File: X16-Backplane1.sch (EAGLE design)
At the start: 29 parts, among them J1 CONN_PXC-8-RA-1778683, J12 282837-3, J13 282837-3, J2 CONN_ET60S-D04-3-08-D04-X-R1-S, J3 HTST-110-04-L-D-RA, J4 CLT-110-01-F-D, U2 TRANS_ULN2003AD

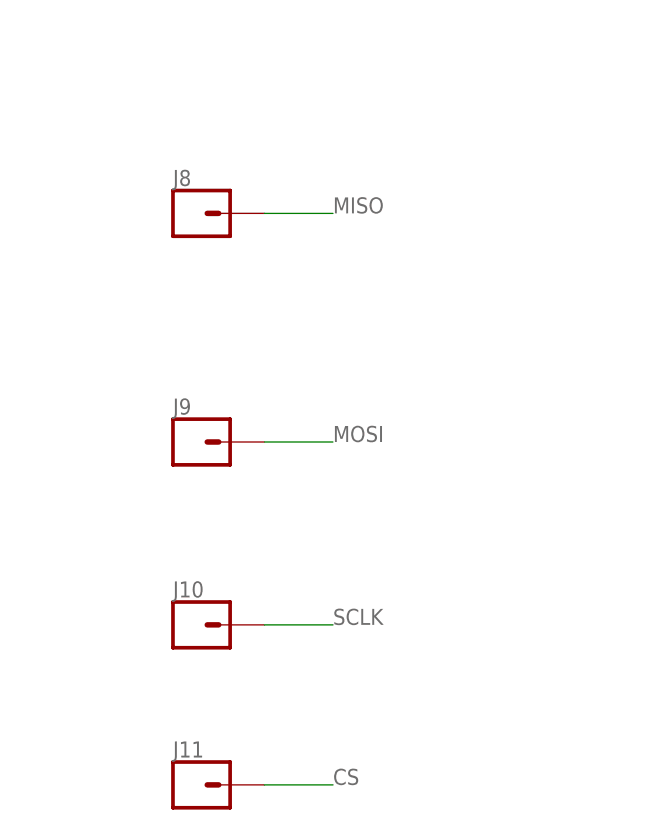
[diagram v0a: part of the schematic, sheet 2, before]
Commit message: Minh Update 3
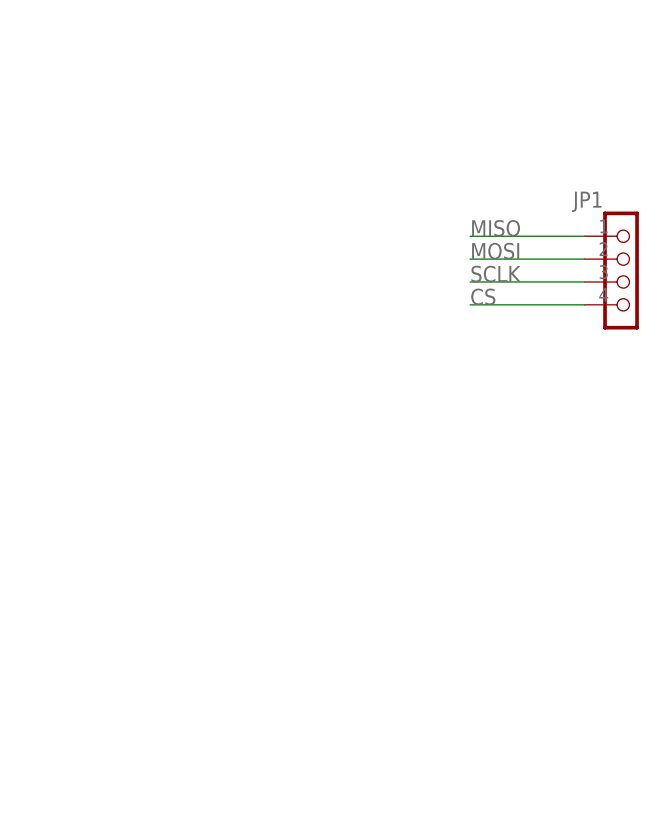
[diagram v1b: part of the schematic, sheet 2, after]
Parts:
- removed J10, J11, J8, J9: (no value), SparkFun-Connectors:CONN_01
- added JP1: (no value), X16-ExtraComponents:TEST_PIN-1X4
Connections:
- net CS: now also JP1.4; no longer J11.1
- net MISO: now also JP1.1; no longer J8.1
- net MOSI: now also JP1.2; no longer J9.1
- net SCLK: now also JP1.3; no longer J10.1
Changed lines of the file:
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@@
 <part name="J3" library="X16_Backplane" deviceset="HTST-110-04-L-D-RA" device=""/>
 <part name="J4" library="X16_Backplane" deviceset="CLT-110-01-F-D" device=""/>
-<part name="J8" library="SparkFun-Connectors" library_urn="urn:adsk.eagle:library:513" deviceset="CONN_01" device="" package3d_urn="urn:adsk.eagle:package:38028/2"/>
-<part name="J9" library="SparkFun-Connectors" library_urn="urn:adsk.eagle:library:513" deviceset="CONN_01" device="" package3d_urn="urn:adsk.eagle:package:38028/2"/>
-<part name="J10" library="SparkFun-Connectors" library_urn="urn:adsk.eagle:library:513" deviceset="CONN_01" device="" package3d_urn="urn:adsk.eagle:package:38028/2"/>
-<part name="J11" library="SparkFun-Connectors" library_urn="urn:adsk.eagle:library:513" deviceset="CONN_01" device="" package3d_urn="urn:adsk.eagle:package:38028/2"/>
 <part name="J12" library="X16_Backplane" deviceset="282837-3" device=""/>
 <part name="J13" library="X16_Backplane" deviceset="282837-3" device=""/>
@@
 <part name="H3" library="X16-ExtraComponents" deviceset="6-32-HOLE" device=""/>
 <part name="H4" library="X16-ExtraComponents" deviceset="6-32-HOLE" device=""/>
+<part name="JP1" library="X16-ExtraComponents" deviceset="TEST_PIN-1X4" device="" package3d_urn="urn:adsk.eagle:package:22407/2"/>
 </parts>
 <sheets>
@@
 <attribute name="C3" x="106.68" y="119.38" size="1.778" layer="96"/>
 </instance>
-<instance part="J8" gate="J1" x="304.8" y="129.54" smashed="yes">
-<attribute name="VALUE" x="302.26" y="124.714" size="1.778" layer="96" font="vector"/>
-<attribute name="NAME" x="302.26" y="132.588" size="1.778" layer="95" font="vector"/>
-</instance>
-<instance part="J9" gate="J1" x="304.8" y="104.14" smashed="yes">
-<attribute name="VALUE" x="302.26" y="99.314" size="1.778" layer="96" font="vector"/>
-<attribute name="NAME" x="302.26" y="107.188" size="1.778" layer="95" font="vector"/>
-</instance>
-<instance part="J10" gate="J1" x="304.8" y="83.82" smashed="yes">
-<attribute name="VALUE" x="302.26" y="78.994" size="1.778" layer="96" font="vector"/>
-<attribute name="NAME" x="302.26" y="86.868" size="1.778" layer="95" font="vector"/>
-</instance>
-<instance part="J11" gate="J1" x="304.8" y="66.04" smashed="yes">
-<attribute name="VALUE" x="302.26" y="61.214" size="1.778" layer="96" font="vector"/>
-<attribute name="NAME" x="302.26" y="69.088" size="1.778" layer="95" font="vector"/>
-</instance>
 <instance part="J12" gate="G$1" x="210.82" y="215.9" smashed="yes">
 <attribute name="NAME" x="207.769640625" y="221.49233125" size="1.27098125" layer="95"/>
@@
 <attribute name="NAME" x="256.54" y="165.1" size="1.016" layer="95" align="bottom-center"/>
 <attribute name="VALUE" x="256.54" y="160.02" size="1.016" layer="95" align="top-center"/>
+</instance>
+<instance part="JP1" gate="A" x="353.06" y="121.92" smashed="yes">
+<attribute name="NAME" x="346.71" y="130.175" size="1.778" layer="95"/>
+<attribute name="VALUE" x="346.71" y="114.3" size="1.778" layer="96"/>
 </instance>
 </instances>
@@
 </segment>
 </net>
-<net name="MISO" class="0">
-<segment>
-<pinref part="J8" gate="J1" pin="1"/>
-<wire x1="312.42" y1="129.54" x2="320.04" y2="129.54" width="0.1524" layer="91"/>
-<label x="320.04" y="129.54" size="1.778" layer="95"/>
-</segment>
-</net>
-<net name="MOSI" class="0">
-<segment>
-<pinref part="J9" gate="J1" pin="1"/>
-<wire x1="312.42" y1="104.14" x2="320.04" y2="104.14" width="0.1524" layer="91"/>
-<label x="320.04" y="104.14" size="1.778" layer="95"/>
-</segment>
-</net>
-<net name="SCLK" class="0">
-<segment>
-<pinref part="J10" gate="J1" pin="1"/>
-<wire x1="312.42" y1="83.82" x2="320.04" y2="83.82" width="0.1524" layer="91"/>
-<label x="320.04" y="83.82" size="1.778" layer="95"/>
-</segment>
-</net>
-<net name="CS" class="0">
-<segment>
-<pinref part="J11" gate="J1" pin="1"/>
-<wire x1="312.42" y1="66.04" x2="320.04" y2="66.04" width="0.1524" layer="91"/>
-<label x="320.04" y="66.04" size="1.778" layer="95"/>
-</segment>
-</net>
 <net name="12V_GND" class="0">
 <segment>
@@
 </segment>
 </net>
+<net name="MISO" class="0">
+<segment>
+<wire x1="347.98" y1="127" x2="335.28" y2="127" width="0.1524" layer="91"/>
+<label x="335.28" y="127" size="1.778" layer="95"/>
+<pinref part="JP1" gate="A" pin="1"/>
+</segment>
+</net>
+<net name="MOSI" class="0">
+<segment>
+<wire x1="347.98" y1="124.46" x2="335.28" y2="124.46" width="0.1524" layer="91"/>
+<label x="335.28" y="124.46" size="1.778" layer="95"/>
+<pinref part="JP1" gate="A" pin="2"/>
+</segment>
+</net>
+<net name="SCLK" class="0">
+<segment>
+<wire x1="347.98" y1="121.92" x2="335.28" y2="121.92" width="0.1524" layer="91"/>
+<label x="335.28" y="121.92" size="1.778" layer="95"/>
+<pinref part="JP1" gate="A" pin="3"/>
+</segment>
+</net>
+<net name="CS" class="0">
+<segment>
+<wire x1="347.98" y1="119.38" x2="335.28" y2="119.38" width="0.1524" layer="91"/>
+<label x="335.28" y="119.38" size="1.778" layer="95"/>
+<pinref part="JP1" gate="A" pin="4"/>
+</segment>
+</net>
